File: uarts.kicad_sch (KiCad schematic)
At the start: 2 parts

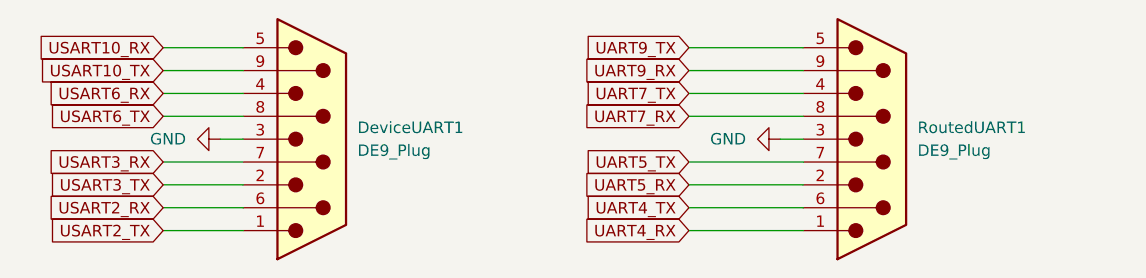
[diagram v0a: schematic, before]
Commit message: uarts routed
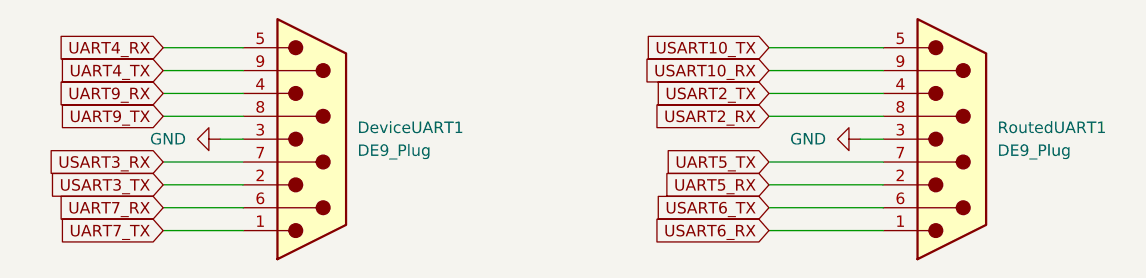
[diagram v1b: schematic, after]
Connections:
- net UART4_RX: now also DeviceUART1.5; no longer RoutedUART1.1
- net UART4_TX: now also DeviceUART1.9; no longer RoutedUART1.6
- net UART7_RX: now also DeviceUART1.6; no longer RoutedUART1.8
- net UART7_TX: now also DeviceUART1.1; no longer RoutedUART1.4
- net UART9_RX: now also DeviceUART1.4; no longer RoutedUART1.9
- net UART9_TX: now also DeviceUART1.8; no longer RoutedUART1.5
- net USART10_RX: now also RoutedUART1.9; no longer DeviceUART1.5
- net USART10_TX: now also RoutedUART1.5; no longer DeviceUART1.9
- net USART2_RX: now also RoutedUART1.8; no longer DeviceUART1.6
- net USART2_TX: now also RoutedUART1.4; no longer DeviceUART1.1
- net USART6_RX: now also RoutedUART1.1; no longer DeviceUART1.4
- net USART6_TX: now also RoutedUART1.6; no longer DeviceUART1.8
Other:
- moved on the sheet: RoutedUART1
